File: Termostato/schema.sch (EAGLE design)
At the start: 11 parts, among them K1 RELAY-SPDT-JZC-11F

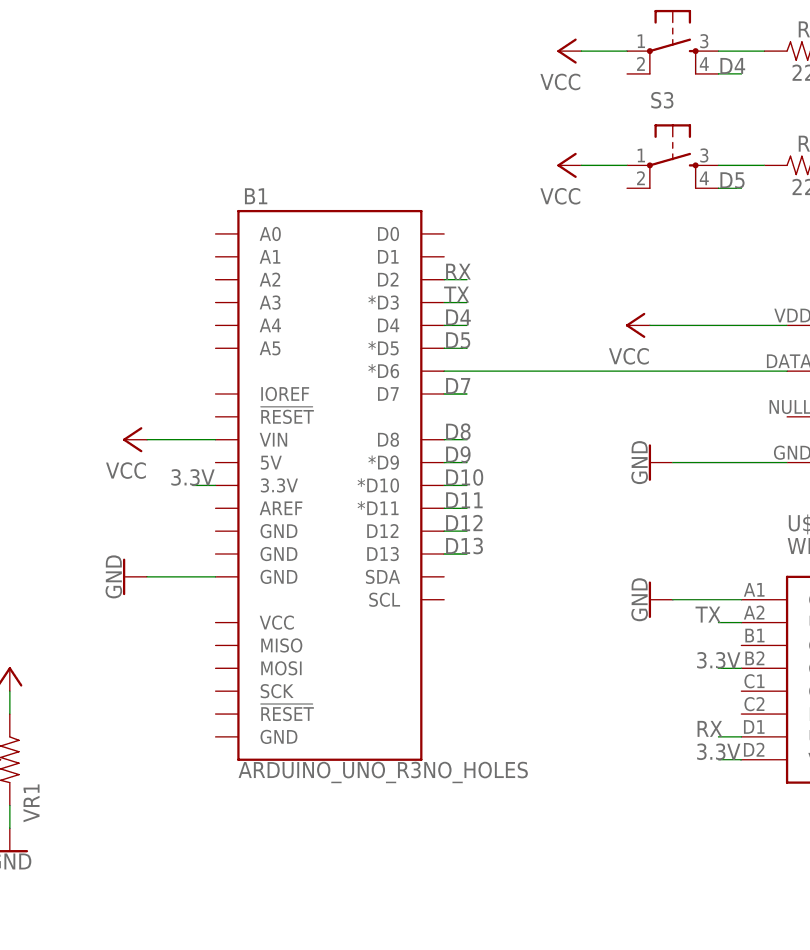
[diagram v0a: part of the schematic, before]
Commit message: Arduino shield
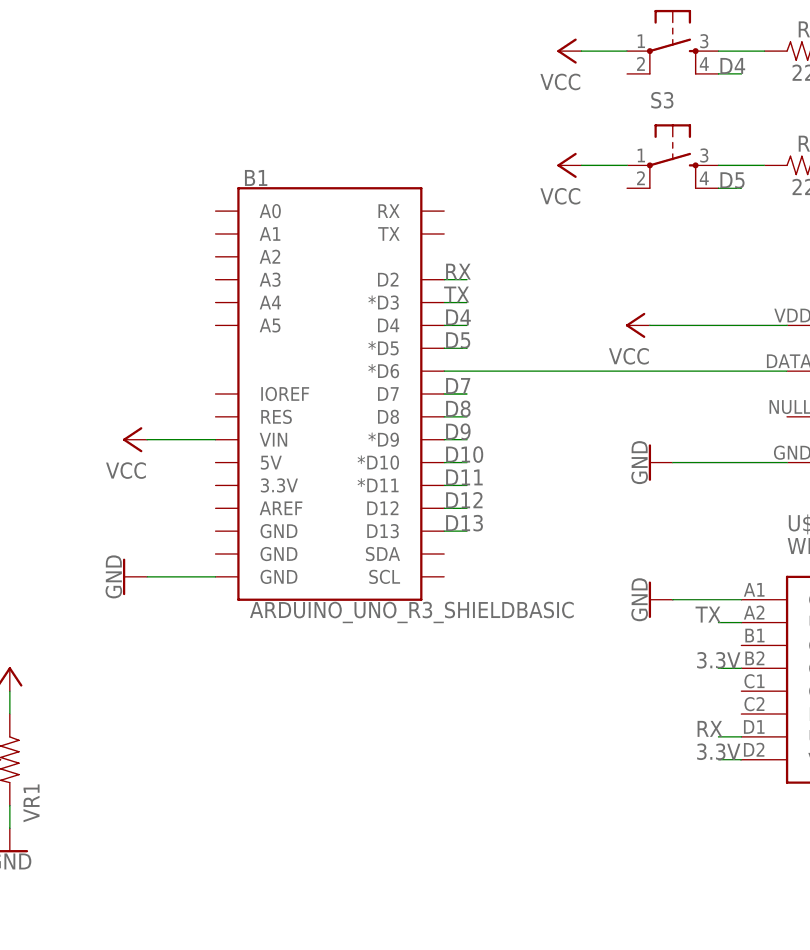
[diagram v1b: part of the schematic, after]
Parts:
- B1: value ARDUINO_UNO_R3NO_HOLES -> ARDUINO_UNO_R3_SHIELDBASIC; device SparkFun-Boards:ARDUINO_UNO_R3NO_HOLES -> SparkFun-Boards:ARDUINO_UNO_R3_SHIELDBASIC
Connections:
- net 3.3V: no longer B1.3.3V
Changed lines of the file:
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@@
 <layers>
 <layer number="1" name="Top" color="4" fill="1" visible="no" active="no"/>
+<layer number="2" name="Route2" color="1" fill="3" visible="no" active="no"/>
+<layer number="3" name="Route3" color="4" fill="3" visible="no" active="no"/>
+<layer number="4" name="Route4" color="1" fill="4" visible="no" active="no"/>
+<layer number="5" name="Route5" color="4" fill="4" visible="no" active="no"/>
+<layer number="6" name="Route6" color="1" fill="8" visible="no" active="no"/>
+<layer number="7" name="Route7" color="4" fill="8" visible="no" active="no"/>
+<layer number="8" name="Route8" color="1" fill="2" visible="no" active="no"/>
+<layer number="9" name="Route9" color="4" fill="2" visible="no" active="no"/>
+<layer number="10" name="Route10" color="1" fill="7" visible="no" active="no"/>
+<layer number="11" name="Route11" color="4" fill="7" visible="no" active="no"/>
+<layer number="12" name="Route12" color="1" fill="5" visible="no" active="no"/>
+<layer number="13" name="Route13" color="4" fill="5" visible="no" active="no"/>
+<layer number="14" name="Route14" color="1" fill="6" visible="no" active="no"/>
+<layer number="15" name="Route15" color="4" fill="6" visible="no" active="no"/>
 <layer number="16" name="Bottom" color="1" fill="1" visible="no" active="no"/>
 <layer number="17" name="Pads" color="2" fill="1" visible="no" active="no"/>
@@
 </classes>
 <parts>
-<part name="B1" library="SparkFun-Boards" deviceset="ARDUINO_UNO_R3" device="NO_HOLES"/>
 <part name="K1" library="SparkFun-Electromechanical" deviceset="RELAY-SPDT" device="-JZC-11F"/>
 <part name="U1" library="RHT03_DHT-22_AM2302" deviceset="RHT03_DHT-22_AM2302" device="RA"/>
@@
 <part name="P+6" library="supply1" library_urn="urn:adsk.eagle:library:371" deviceset="VCC" device=""/>
 <part name="P+7" library="supply1" library_urn="urn:adsk.eagle:library:371" deviceset="VCC" device=""/>
+<part name="B1" library="SparkFun-Boards" deviceset="ARDUINO_UNO_R3_SHIELD" device="BASIC"/>
 </parts>
 <sheets>
@@
 </plain>
 <instances>
-<instance part="B1" gate="G$1" x="71.12" y="116.84"/>
 <instance part="K1" gate="K$1" x="2.54" y="142.24" rot="R180"/>
 <instance part="U1" gate="G$1" x="132.08" y="127"/>
@@
 <instance part="P+6" gate="VCC" x="96.52" y="152.4" rot="R90"/>
 <instance part="P+7" gate="VCC" x="96.52" y="165.1" rot="R90"/>
+<instance part="B1" gate="G$1" x="71.12" y="129.54"/>
 </instances>
 <busses>
@@
 <segment>
 <pinref part="GND4" gate="1" pin="GND"/>
+<wire x1="50.8" y1="106.68" x2="58.42" y2="106.68" width="0.1524" layer="91"/>
 <pinref part="B1" gate="G$1" pin="GND@0"/>
-<wire x1="50.8" y1="106.68" x2="58.42" y2="106.68" width="0.1524" layer="91"/>
 </segment>
 <segment>
@@
 <segment>
 <pinref part="P+3" gate="VCC" pin="VCC"/>
+<wire x1="50.8" y1="121.92" x2="58.42" y2="121.92" width="0.1524" layer="91"/>
 <pinref part="B1" gate="G$1" pin="VIN"/>
-<wire x1="50.8" y1="121.92" x2="58.42" y2="121.92" width="0.1524" layer="91"/>
 </segment>
 <segment>
@@
 <net name="N$3" class="0">
 <segment>
-<pinref part="B1" gate="G$1" pin="*D6"/>
 <pinref part="U1" gate="G$1" pin="DATA"/>
 <wire x1="83.82" y1="129.54" x2="121.92" y2="129.54" width="0.1524" layer="91"/>
+<pinref part="B1" gate="G$1" pin="*D6"/>
 </segment>
 </net>
 <net name="D7" class="0">
 <segment>
-<pinref part="B1" gate="G$1" pin="D7"/>
 <wire x1="83.82" y1="127" x2="86.36" y2="127" width="0.1524" layer="91"/>
 <label x="83.82" y="127" size="1.778" layer="95"/>
+<pinref part="B1" gate="G$1" pin="D7"/>
 </segment>
 <segment>
@@
 </segment>
 <segment>
-<pinref part="B1" gate="G$1" pin="*D3"/>
 <wire x1="83.82" y1="137.16" x2="86.36" y2="137.16" width="0.1524" layer="91"/>
 <label x="83.82" y="137.16" size="1.778" layer="95"/>
+<pinref part="B1" gate="G$1" pin="*D3"/>
 </segment>
 </net>
@@
 </segment>
 <segment>
-<pinref part="B1" gate="G$1" pin="D2"/>
 <wire x1="83.82" y1="139.7" x2="86.36" y2="139.7" width="0.1524" layer="91"/>
 <label x="83.82" y="139.7" size="1.778" layer="95"/>
+<pinref part="B1" gate="G$1" pin="D2"/>
 </segment>
 </net>
@@
 </segment>
 <segment>
-<pinref part="B1" gate="G$1" pin="3.3V"/>
-<wire x1="58.42" y1="116.84" x2="55.88" y2="116.84" width="0.1524" layer="91"/>
-<label x="53.34" y="116.84" size="1.778" layer="95"/>
-</segment>
-<segment>
 <pinref part="U$1" gate="G$1" pin="CH_PD"/>
 <wire x1="116.84" y1="96.52" x2="114.3" y2="96.52" width="0.1524" layer="91"/>
@@
 <segment>
 <pinref part="B1" gate="G$1" pin="D13"/>
-<wire x1="83.82" y1="109.22" x2="86.36" y2="109.22" width="0.1524" layer="91"/>
-<label x="83.82" y="109.22" size="1.778" layer="95"/>
+<wire x1="83.82" y1="111.76" x2="86.36" y2="111.76" width="0.1524" layer="91"/>
+<label x="83.82" y="111.76" size="1.778" layer="95"/>
 </segment>
 </net>
@@
 <segment>
 <pinref part="B1" gate="G$1" pin="D8"/>
-<wire x1="83.82" y1="121.92" x2="86.36" y2="121.92" width="0.1524" layer="91"/>
-<label x="83.82" y="121.92" size="1.778" layer="95"/>
+<wire x1="83.82" y1="124.46" x2="86.36" y2="124.46" width="0.1524" layer="91"/>
+<label x="83.82" y="124.46" size="1.778" layer="95"/>
 </segment>
 </net>
@@
 <segment>
 <pinref part="B1" gate="G$1" pin="*D9"/>
-<wire x1="83.82" y1="119.38" x2="86.36" y2="119.38" width="0.1524" layer="91"/>
-<label x="83.82" y="119.38" size="1.778" layer="95"/>
+<wire x1="83.82" y1="121.92" x2="86.36" y2="121.92" width="0.1524" layer="91"/>
+<label x="83.82" y="121.92" size="1.778" layer="95"/>
 </segment>
 </net>
@@
 <segment>
 <pinref part="B1" gate="G$1" pin="*D10"/>
-<wire x1="83.82" y1="116.84" x2="86.36" y2="116.84" width="0.1524" layer="91"/>
-<label x="83.82" y="116.84" size="1.778" layer="95"/>
+<wire x1="83.82" y1="119.38" x2="86.36" y2="119.38" width="0.1524" layer="91"/>
+<label x="83.82" y="119.38" size="1.778" layer="95"/>
 </segment>
 </net>
@@
 <segment>
 <pinref part="B1" gate="G$1" pin="*D11"/>
-<wire x1="83.82" y1="114.3" x2="86.36" y2="114.3" width="0.1524" layer="91"/>
-<label x="83.82" y="114.3" size="1.778" layer="95"/>
+<wire x1="83.82" y1="116.84" x2="86.36" y2="116.84" width="0.1524" layer="91"/>
+<label x="83.82" y="116.84" size="1.778" layer="95"/>
 </segment>
 </net>
@@
 <segment>
 <pinref part="B1" gate="G$1" pin="D12"/>
-<wire x1="83.82" y1="111.76" x2="86.36" y2="111.76" width="0.1524" layer="91"/>
-<label x="83.82" y="111.76" size="1.778" layer="95"/>
+<wire x1="83.82" y1="114.3" x2="86.36" y2="114.3" width="0.1524" layer="91"/>
+<label x="83.82" y="114.3" size="1.778" layer="95"/>
 </segment>
 </net>
@@
 </segment>
 <segment>
-<pinref part="B1" gate="G$1" pin="D4"/>
 <wire x1="83.82" y1="134.62" x2="86.36" y2="134.62" width="0.1524" layer="91"/>
 <label x="83.82" y="134.62" size="1.778" layer="95"/>
+<pinref part="B1" gate="G$1" pin="D4"/>
 </segment>
 </net>
@@
 </segment>
 <segment>
-<pinref part="B1" gate="G$1" pin="*D5"/>
 <wire x1="83.82" y1="132.08" x2="86.36" y2="132.08" width="0.1524" layer="91"/>
 <label x="83.82" y="132.08" size="1.778" layer="95"/>
-</segment>
-</net>
+<pinref part="B1" gate="G$1" pin="*D5"/>
+</segment>
+</net>
